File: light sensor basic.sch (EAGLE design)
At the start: 2 parts, among them U1 VCNT2020

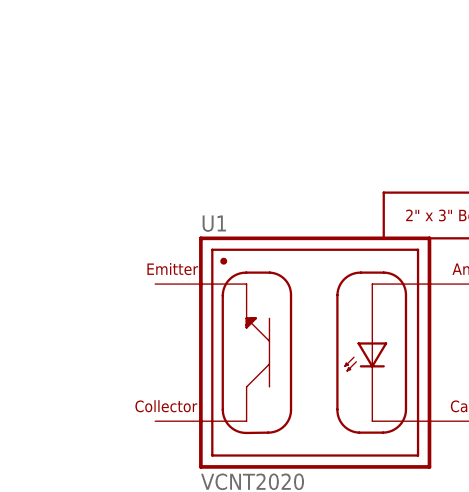
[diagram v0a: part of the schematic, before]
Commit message: wont change
github schematic absolutely refuses to update
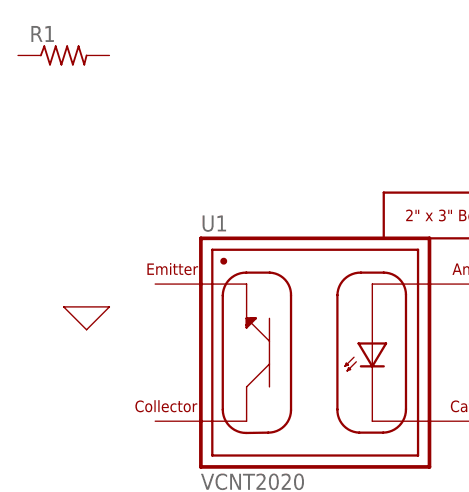
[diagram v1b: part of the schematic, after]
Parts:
- added R1: (no value), rcl:R-US_R1206
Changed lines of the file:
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@@
 <part name="U$1" library="voltera_community_lib" deviceset="2X3_BOARD" device="_V2"/>
 <part name="U1" library="VCNT2020" deviceset="VCNT2020" device=""/>
+<part name="R1" library="rcl" library_urn="urn:adsk.eagle:library:334" deviceset="R-US_" device="R1206" package3d_urn="urn:adsk.eagle:package:23540/2"/>
+<part name="X_1" library="ngspice-simulation" library_urn="urn:adsk.eagle:library:527439" deviceset="GND" device=""/>
 </parts>
 <sheets>
@@
 <attribute name="VALUE" x="-2.54" y="-5.08" size="1.778" layer="96"/>
 </instance>
+<instance part="R1" gate="G$1" x="-17.78" y="43.18" smashed="yes">
+<attribute name="NAME" x="-21.59" y="44.6786" size="1.778" layer="95"/>
+<attribute name="VALUE" x="-21.59" y="39.878" size="1.778" layer="96"/>
+</instance>
+<instance part="X_1" gate="G$1" x="-15.24" y="15.24" smashed="yes"/>
 </instances>
 <busses>
@@
 </schematic>
 </drawing>
+<compatibility>
+<note version="8.2" severity="warning">
+Since Version 8.2, EAGLE supports online libraries. The ids
+of those online libraries will not be understood (or retained)
+with this version.
+</note>
+<note version="8.3" severity="warning">
+Since Version 8.3, EAGLE supports URNs for individual library
+assets (packages, symbols, and devices). The URNs of those assets
+will not be understood (or retained) with this version.
+</note>
+<note version="8.3" severity="warning">
+Since Version 8.3, EAGLE supports the association of 3D packages
+with devices in libraries, schematics, and board files. Those 3D
+packages will not be understood (or retained) with this version.
+</note>
+<note version="8.4" severity="warning">
+Since Version 8.4, EAGLE supports properties for SPICE simulation.
+Probes in schematics and SPICE mapping objects found in parts and library devices
+will not be understood with this version. Update EAGLE to the latest version
+for full support of SPICE simulation.
+</note>
+</compatibility>
 </eagle>

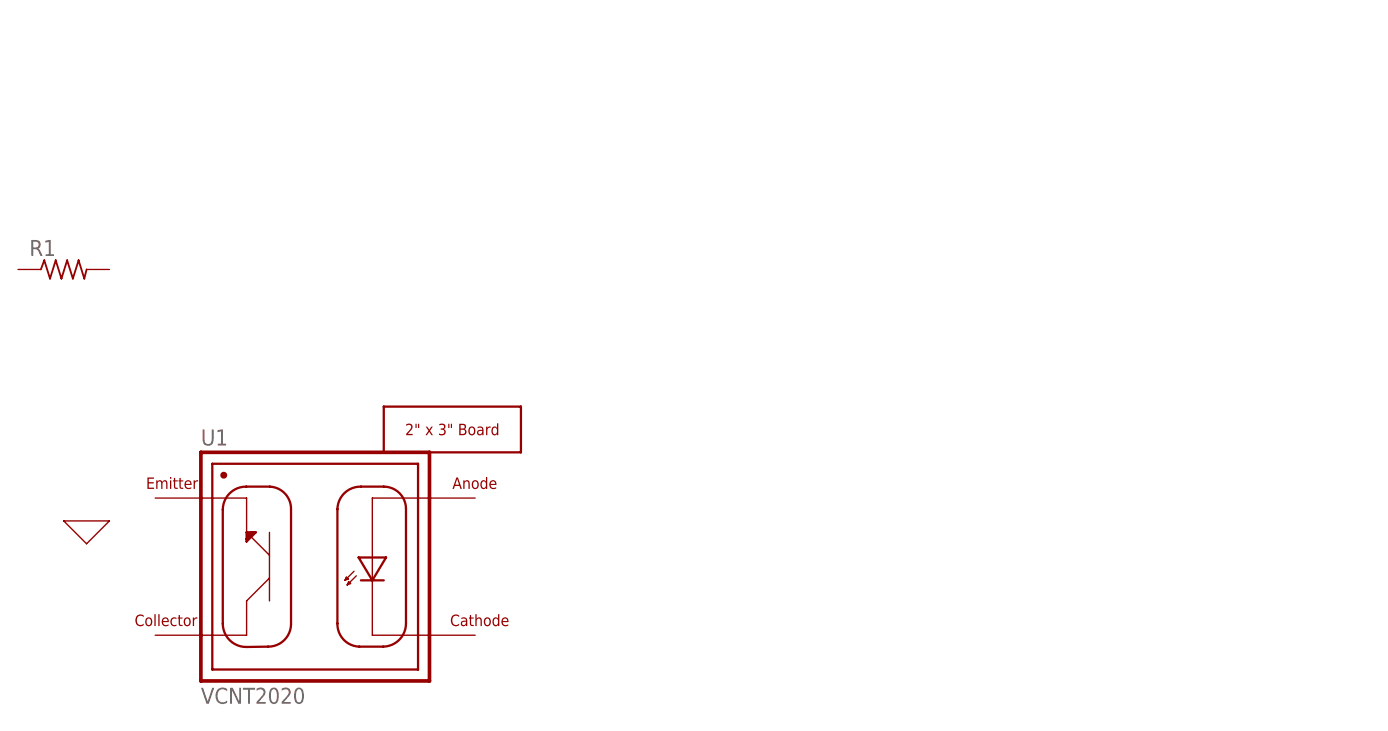
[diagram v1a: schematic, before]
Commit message: SHOULD WORK
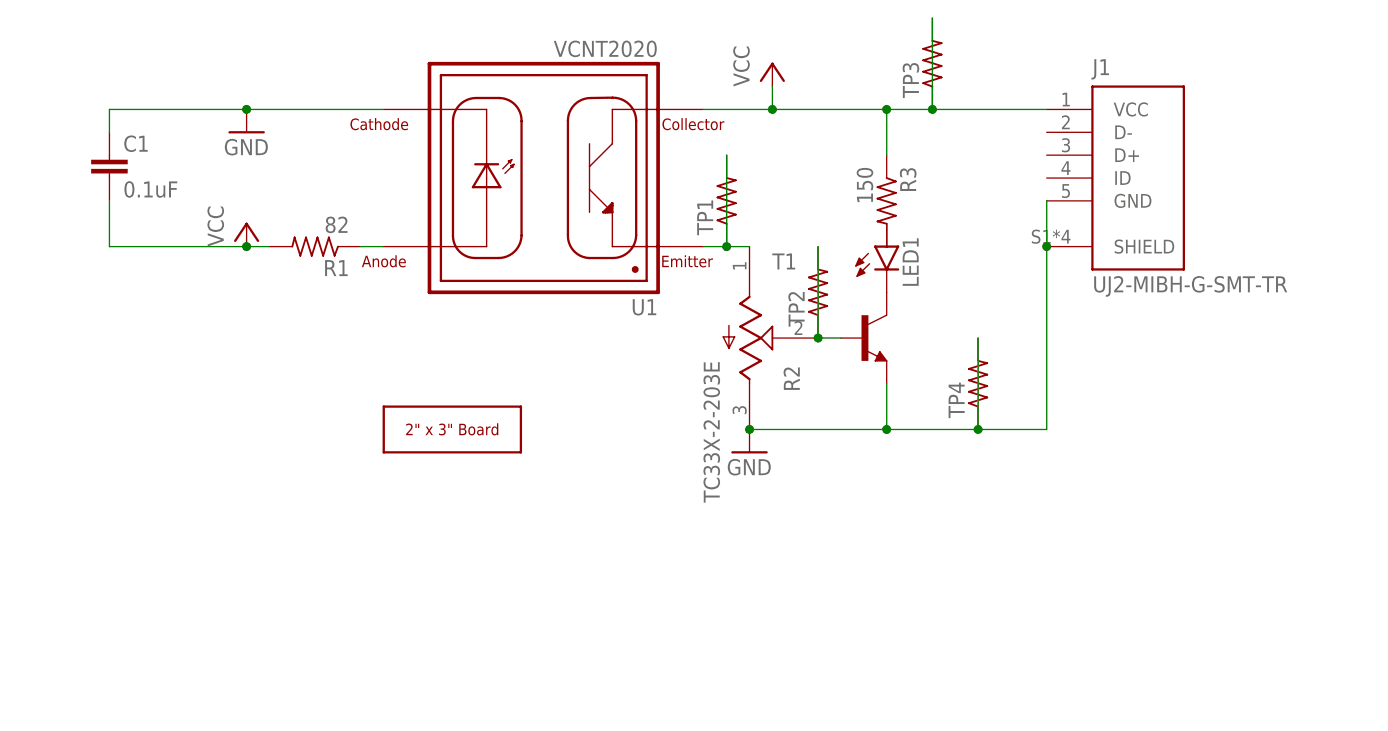
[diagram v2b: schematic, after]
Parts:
- added C1: 0.1uF, rcl:C-EUC1206
- added J1: UJ2-MIBH-G-SMT-TR, UJ2-MIBH-G-SMT-TR:UJ2-MIBH-G-SMT-TR
- added LED1: (no value), led:LEDSML0805
- added R2: TC33X-2-203E, TC33X-2-203E:TC33X-2-203E
- added R3: 150, rcl:R-US_R0805
- added T1: (no value), transistor:-NPN-SOT23-EBC
- added TP1, TP2, TP3, TP4: (no value), rcl:R-US_R1206
- R1: value (none) -> 82; device rcl:R-US_R1206 -> rcl:R-US_R0805
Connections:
- new net GND: C1.1, J1.GND, J1.SHIELD, R2.CW, T1.E, TP4.1, TP4.2, U1.CATHODE
- new net N$1: R1.1, U1.ANODE
- new net N$2: R2.CCW, TP1.1, TP1.2, U1.EMITTER
- new net N$3: R2.W, T1.B, TP2.1, TP2.2
- new net N$4: LED1.C, T1.C
- new net VCC: C1.2, J1.VCC, R1.2, R3.1, TP3.1, TP3.2, U1.COLLECTOR
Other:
- moved on the sheet: R1, U1

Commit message: c
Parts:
- R1: device rcl:R-US_R0805 -> rcl:R-US_R1206
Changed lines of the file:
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@@
 <grid distance="0.1" unitdist="inch" unit="inch" style="lines" multiple="1" display="no" altdistance="0.01" altunitdist="inch" altunit="inch"/>
 <layers>
-<layer number="1" name="Top" color="4" fill="1" visible="no" active="no"/>
-<layer number="2" name="Route2" color="1" fill="3" visible="no" active="no"/>
-<layer number="3" name="Route3" color="4" fill="3" visible="no" active="no"/>
-<layer number="4" name="Route4" color="1" fill="4" visible="no" active="no"/>
-<layer number="5" name="Route5" color="4" fill="4" visible="no" active="no"/>
-<layer number="6" name="Route6" color="1" fill="8" visible="no" active="no"/>
-<layer number="7" name="Route7" color="4" fill="8" visible="no" active="no"/>
-<layer number="8" name="Route8" color="1" fill="2" visible="no" active="no"/>
-<layer number="9" name="Route9" color="4" fill="2" visible="no" active="no"/>
-<layer number="10" name="Route10" color="1" fill="7" visible="no" active="no"/>
-<layer number="11" name="Route11" color="4" fill="7" visible="no" active="no"/>
-<layer number="12" name="Route12" color="1" fill="5" visible="no" active="no"/>
-<layer number="13" name="Route13" color="4" fill="5" visible="no" active="no"/>
-<layer number="14" name="Route14" color="1" fill="6" visible="no" active="no"/>
-<layer number="15" name="Route15" color="4" fill="6" visible="no" active="no"/>
-<layer number="16" name="Bottom" color="1" fill="1" visible="no" active="no"/>
-<layer number="17" name="Pads" color="2" fill="1" visible="no" active="no"/>
-<layer number="18" name="Vias" color="2" fill="1" visible="no" active="no"/>
-<layer number="19" name="Unrouted" color="6" fill="1" visible="no" active="no"/>
-<layer number="20" name="Dimension" color="15" fill="1" visible="no" active="no"/>
-<layer number="21" name="tPlace" color="7" fill="1" visible="no" active="no"/>
-<layer number="22" name="bPlace" color="7" fill="1" visible="no" active="no"/>
-<layer number="23" name="tOrigins" color="15" fill="1" visible="no" active="no"/>
-<layer number="24" name="bOrigins" color="15" fill="1" visible="no" active="no"/>
-<layer number="25" name="tNames" color="7" fill="1" visible="no" active="no"/>
-<layer number="26" name="bNames" color="7" fill="1" visible="no" active="no"/>
-<layer number="27" name="tValues" color="7" fill="1" visible="no" active="no"/>
-<layer number="28" name="bValues" color="7" fill="1" visible="no" active="no"/>
+<layer number="1" name="Top" color="4" fill="1" visible="yes" active="no"/>
+<layer number="2" name="Route2" color="16" fill="1" visible="yes" active="no"/>
+<layer number="3" name="Route3" color="17" fill="1" visible="yes" active="no"/>
+<layer number="4" name="Route4" color="18" fill="1" visible="yes" active="no"/>
+<layer number="5" name="Route5" color="19" fill="1" visible="yes" active="no"/>
+<layer number="6" name="Route6" color="25" fill="1" visible="yes" active="no"/>
+<layer number="7" name="Route7" color="26" fill="1" visible="yes" active="no"/>
+<layer number="8" name="Route8" color="27" fill="1" visible="yes" active="no"/>
+<layer number="9" name="Route9" color="28" fill="1" visible="yes" active="no"/>
+<layer number="10" name="Route10" color="29" fill="1" visible="yes" active="no"/>
+<layer number="11" name="Route11" color="30" fill="1" visible="yes" active="no"/>
+<layer number="12" name="Route12" color="20" fill="1" visible="yes" active="no"/>
+<layer number="13" name="Route13" color="21" fill="1" visible="yes" active="no"/>
+<layer number="14" name="Route14" color="22" fill="1" visible="yes" active="no"/>
+<layer number="15" name="Route15" color="23" fill="1" visible="yes" active="no"/>
+<layer number="16" name="Bottom" color="1" fill="1" visible="yes" active="no"/>
+<layer number="17" name="Pads" color="2" fill="1" visible="yes" active="no"/>
+<layer number="18" name="Vias" color="2" fill="1" visible="yes" active="no"/>
+<layer number="19" name="Unrouted" color="6" fill="1" visible="yes" active="no"/>
+<layer number="20" name="Dimension" color="24" fill="1" visible="yes" active="no"/>
+<layer number="21" name="tPlace" color="7" fill="1" visible="yes" active="no"/>
+<layer number="22" name="bPlace" color="7" fill="1" visible="yes" active="no"/>
+<layer number="23" name="tOrigins" color="15" fill="1" visible="yes" active="no"/>
+<layer number="24" name="bOrigins" color="15" fill="1" visible="yes" active="no"/>
+<layer number="25" name="tNames" color="7" fill="1" visible="yes" active="no"/>
+<layer number="26" name="bNames" color="7" fill="1" visible="yes" active="no"/>
+<layer number="27" name="tValues" color="7" fill="1" visible="yes" active="no"/>
+<layer number="28" name="bValues" color="7" fill="1" visible="yes" active="no"/>
 <layer number="29" name="tStop" color="7" fill="3" visible="no" active="no"/>
 <layer number="30" name="bStop" color="7" fill="6" visible="no" active="no"/>
@@
 <layer number="35" name="tGlue" color="7" fill="4" visible="no" active="no"/>
 <layer number="36" name="bGlue" color="7" fill="5" visible="no" active="no"/>
-<layer number="37" name="tTest" color="7" fill="1" visible="no" active="no"/>
-<layer number="38" name="bTest" color="7" fill="1" visible="no" active="no"/>
+<layer number="37" name="tTest" color="7" fill="1" visible="yes" active="no"/>
+<layer number="38" name="bTest" color="7" fill="1" visible="yes" active="no"/>
 <layer number="39" name="tKeepout" color="4" fill="11" visible="no" active="no"/>
 <layer number="40" name="bKeepout" color="1" fill="11" visible="no" active="no"/>
@@
 <layer number="44" name="Drills" color="7" fill="1" visible="no" active="no"/>
 <layer number="45" name="Holes" color="7" fill="1" visible="no" active="no"/>
-<layer number="46" name="Milling" color="3" fill="1" visible="no" active="no"/>
-<layer number="47" name="Measures" color="7" fill="1" visible="no" active="no"/>
-<layer number="48" name="Document" color="7" fill="1" visible="no" active="no"/>
-<layer number="49" name="Reference" color="7" fill="1" visible="no" active="no"/>
-<layer number="50" name="dxf" color="7" fill="1" visible="no" active="no"/>
-<layer number="51" name="tDocu" color="7" fill="1" visible="no" active="no"/>
-<layer number="52" name="bDocu" color="7" fill="1" visible="no" active="no"/>
-<layer number="53" name="tGND_GNDA" color="7" fill="9" visible="no" active="no"/>
-<layer number="54" name="bGND_GNDA" color="1" fill="9" visible="no" active="no"/>
-<layer number="56" name="wert" color="7" fill="1" visible="no" active="no"/>
-<layer number="57" name="tCAD" color="7" fill="1" visible="no" active="no"/>
-<layer number="58" name="bCAD" color="7" fill="1" visible="no" active="no"/>
-<layer number="59" name="tCarbon" color="7" fill="1" visible="no" active="no"/>
-<layer number="60" name="bCarbon" color="7" fill="1" visible="no" active="no"/>
+<layer number="46" name="Milling" color="3" fill="1" visible="yes" active="no"/>
+<layer number="47" name="Measures" color="7" fill="1" visible="yes" active="no"/>
+<layer number="48" name="Document" color="7" fill="1" visible="yes" active="no"/>
+<layer number="49" name="Reference" color="7" fill="1" visible="yes" active="no"/>
+<layer number="50" name="dxf" color="7" fill="1" visible="yes" active="no"/>
+<layer number="51" name="tDocu" color="7" fill="1" visible="yes" active="no"/>
+<layer number="52" name="bDocu" color="7" fill="1" visible="yes" active="no"/>
+<layer number="53" name="tGND_GNDA" color="7" fill="9" visible="yes" active="no"/>
+<layer number="54" name="bGND_GNDA" color="1" fill="9" visible="yes" active="no"/>
+<layer number="56" name="wert" color="7" fill="1" visible="yes" active="no"/>
+<layer number="57" name="tCAD" color="7" fill="1" visible="yes" active="no"/>
+<layer number="58" name="bCAD" color="7" fill="1" visible="yes" active="no"/>
+<layer number="59" name="tCarbon" color="7" fill="1" visible="yes" active="no"/>
+<layer number="60" name="bCarbon" color="7" fill="1" visible="yes" active="no"/>
 <layer number="88" name="SimResults" color="9" fill="1" visible="yes" active="yes"/>
 <layer number="89" name="SimProbes" color="9" fill="1" visible="yes" active="yes"/>
@@
 <part name="U1" library="VCNT2020" deviceset="VCNT2020" device=""/>
 <part name="P+1" library="supply1" library_urn="urn:adsk.eagle:library:371" deviceset="VCC" device=""/>
-<part name="R1" library="rcl" library_urn="urn:adsk.eagle:library:334" deviceset="R-US_" device="R0805" package3d_urn="urn:adsk.eagle:package:23553/2" value="82"/>
+<part name="R1" library="rcl" library_urn="urn:adsk.eagle:library:334" deviceset="R-US_" device="R1206" package3d_urn="urn:adsk.eagle:package:23540/2" value="82"/>
 <part name="GND1" library="supply1" library_urn="urn:adsk.eagle:library:371" deviceset="GND" device=""/>
 <part name="C1" library="rcl" library_urn="urn:adsk.eagle:library:334" deviceset="C-EU" device="C1206" package3d_urn="urn:adsk.eagle:package:23618/2" value="0.1uF"/>

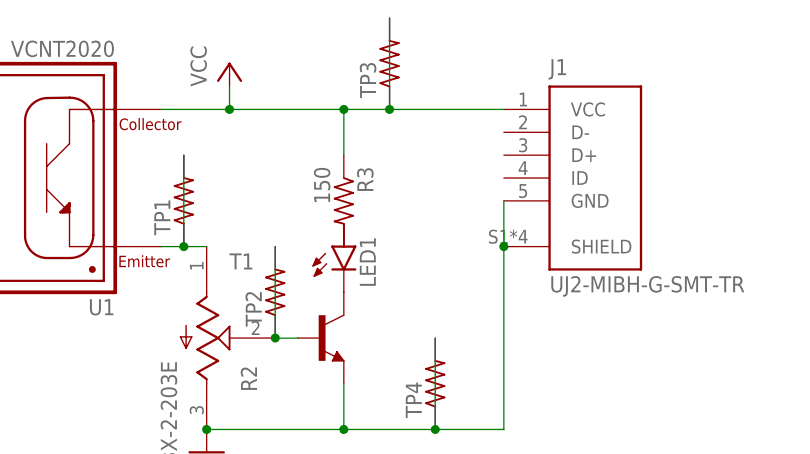
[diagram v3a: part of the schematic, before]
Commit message: a
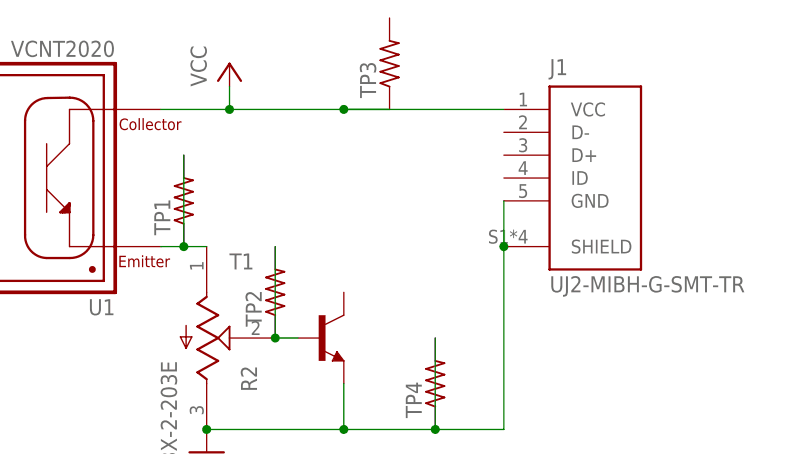
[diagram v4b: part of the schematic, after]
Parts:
- removed LED1: (no value), led:LEDSML0805
- removed R3: 150, rcl:R-US_R0805
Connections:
- removed net N$4: LED1.C, T1.C
- net VCC: no longer R3.1, TP3.2
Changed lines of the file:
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@@
 <part name="GND2" library="supply1" library_urn="urn:adsk.eagle:library:371" deviceset="GND" device=""/>
 <part name="T1" library="transistor" library_urn="urn:adsk.eagle:library:402" deviceset="*-NPN-" device="SOT23-EBC" package3d_urn="urn:adsk.eagle:package:28750/3"/>
-<part name="LED1" library="led" library_urn="urn:adsk.eagle:library:259" deviceset="LED" device="SML0805" package3d_urn="urn:adsk.eagle:package:15830/1"/>
-<part name="R3" library="rcl" library_urn="urn:adsk.eagle:library:334" deviceset="R-US_" device="R0805" package3d_urn="urn:adsk.eagle:package:23553/2" value="150"/>
 <part name="J1" library="UJ2-MIBH-G-SMT-TR" deviceset="UJ2-MIBH-G-SMT-TR" device=""/>
 <part name="TP3" library="rcl" library_urn="urn:adsk.eagle:library:334" deviceset="R-US_" device="R1206" package3d_urn="urn:adsk.eagle:package:23540/2"/>
@@
 <attribute name="NAME" x="60.96" y="43.18" size="1.778" layer="95"/>
 <attribute name="VALUE" x="60.96" y="40.64" size="1.778" layer="96"/>
-</instance>
-<instance part="LED1" gate="G$1" x="73.66" y="45.72" smashed="yes">
-<attribute name="NAME" x="77.216" y="41.148" size="1.778" layer="95" rot="R90"/>
-<attribute name="VALUE" x="79.375" y="41.148" size="1.778" layer="96" rot="R90"/>
-</instance>
-<instance part="R3" gate="G$1" x="73.66" y="50.8" smashed="yes" rot="R270">
-<attribute name="NAME" x="75.1586" y="54.61" size="1.778" layer="95" rot="R270"/>
-<attribute name="VALUE" x="70.358" y="54.61" size="1.778" layer="96" rot="R270"/>
 </instance>
 <instance part="J1" gate="G$1" x="101.6" y="53.34" smashed="yes">
@@
 <wire x1="60.96" y1="60.96" x2="73.66" y2="60.96" width="0.1524" layer="91"/>
 <junction x="60.96" y="60.96"/>
-<pinref part="R3" gate="G$1" pin="1"/>
-<wire x1="73.66" y1="60.96" x2="73.66" y2="55.88" width="0.1524" layer="91"/>
 <pinref part="J1" gate="G$1" pin="VCC"/>
+<pinref part="TP3" gate="G$1" pin="1"/>
+<wire x1="73.66" y1="60.96" x2="91.44" y2="60.96" width="0.1524" layer="91"/>
+<junction x="73.66" y="60.96"/>
 <wire x1="73.66" y1="60.96" x2="78.74" y2="60.96" width="0.1524" layer="91"/>
-<junction x="73.66" y="60.96"/>
-<pinref part="TP3" gate="G$1" pin="1"/>
-<wire x1="78.74" y1="60.96" x2="91.44" y2="60.96" width="0.1524" layer="91"/>
-<junction x="78.74" y="60.96"/>
-<pinref part="TP3" gate="G$1" pin="2"/>
-<wire x1="78.74" y1="71.12" x2="78.74" y2="60.96" width="0.1524" layer="91"/>
 </segment>
 </net>
@@
 </segment>
 </net>
-<net name="N$4" class="0">
-<segment>
-<pinref part="T1" gate="G$1" pin="C"/>
-<pinref part="LED1" gate="G$1" pin="C"/>
-</segment>
-</net>
